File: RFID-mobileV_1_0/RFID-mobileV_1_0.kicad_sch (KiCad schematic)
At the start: 24 parts

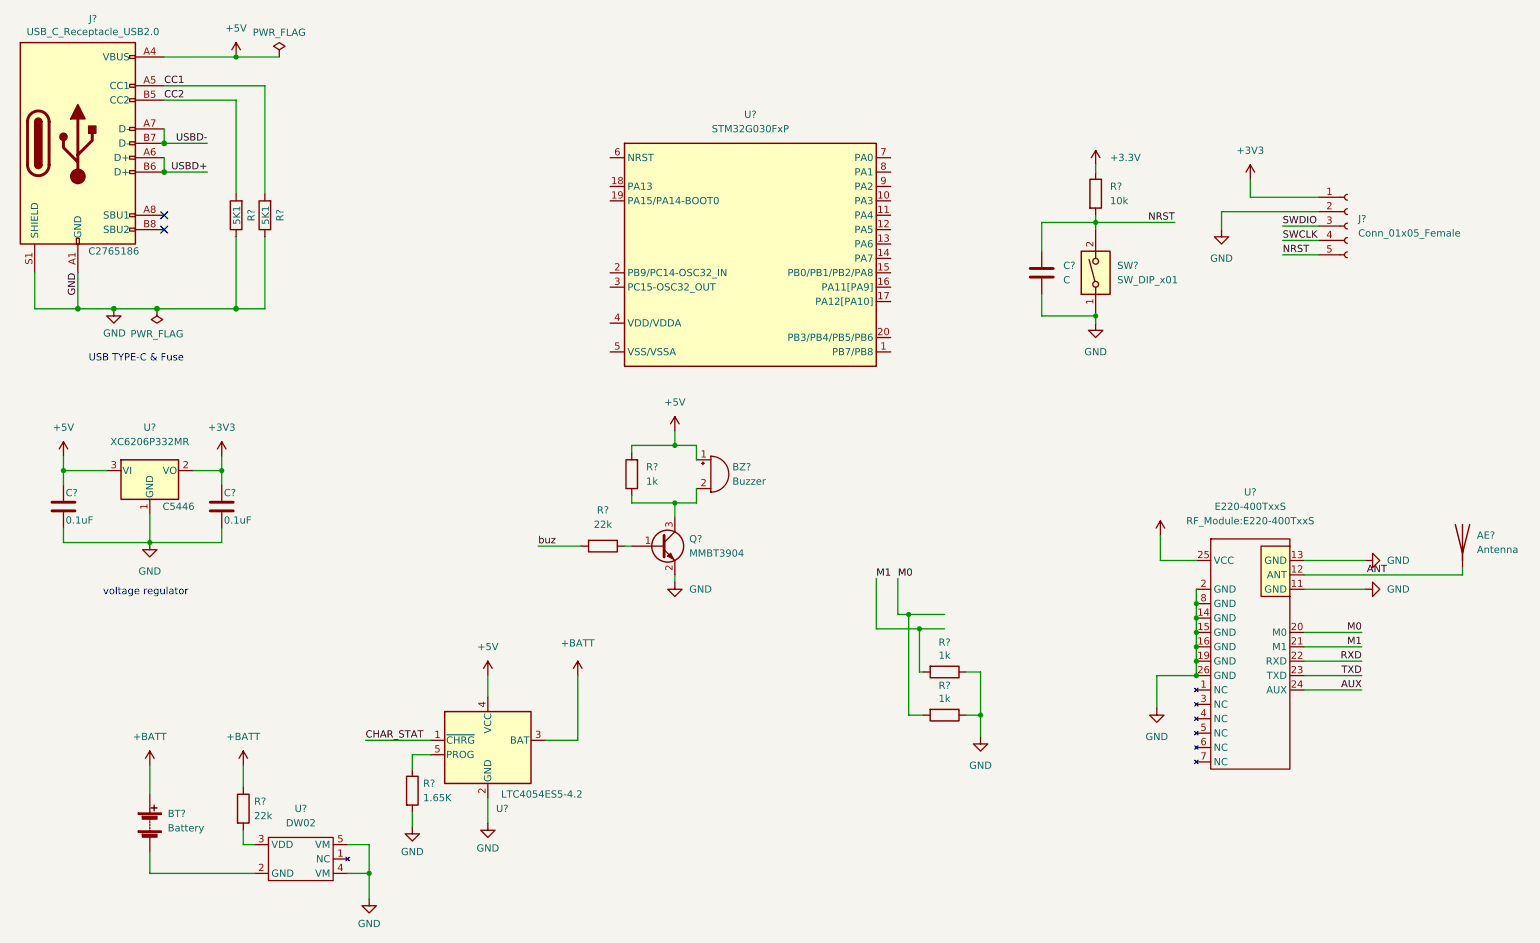
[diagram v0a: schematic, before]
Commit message: Update RFID-mobileV_1_0.kicad_sch
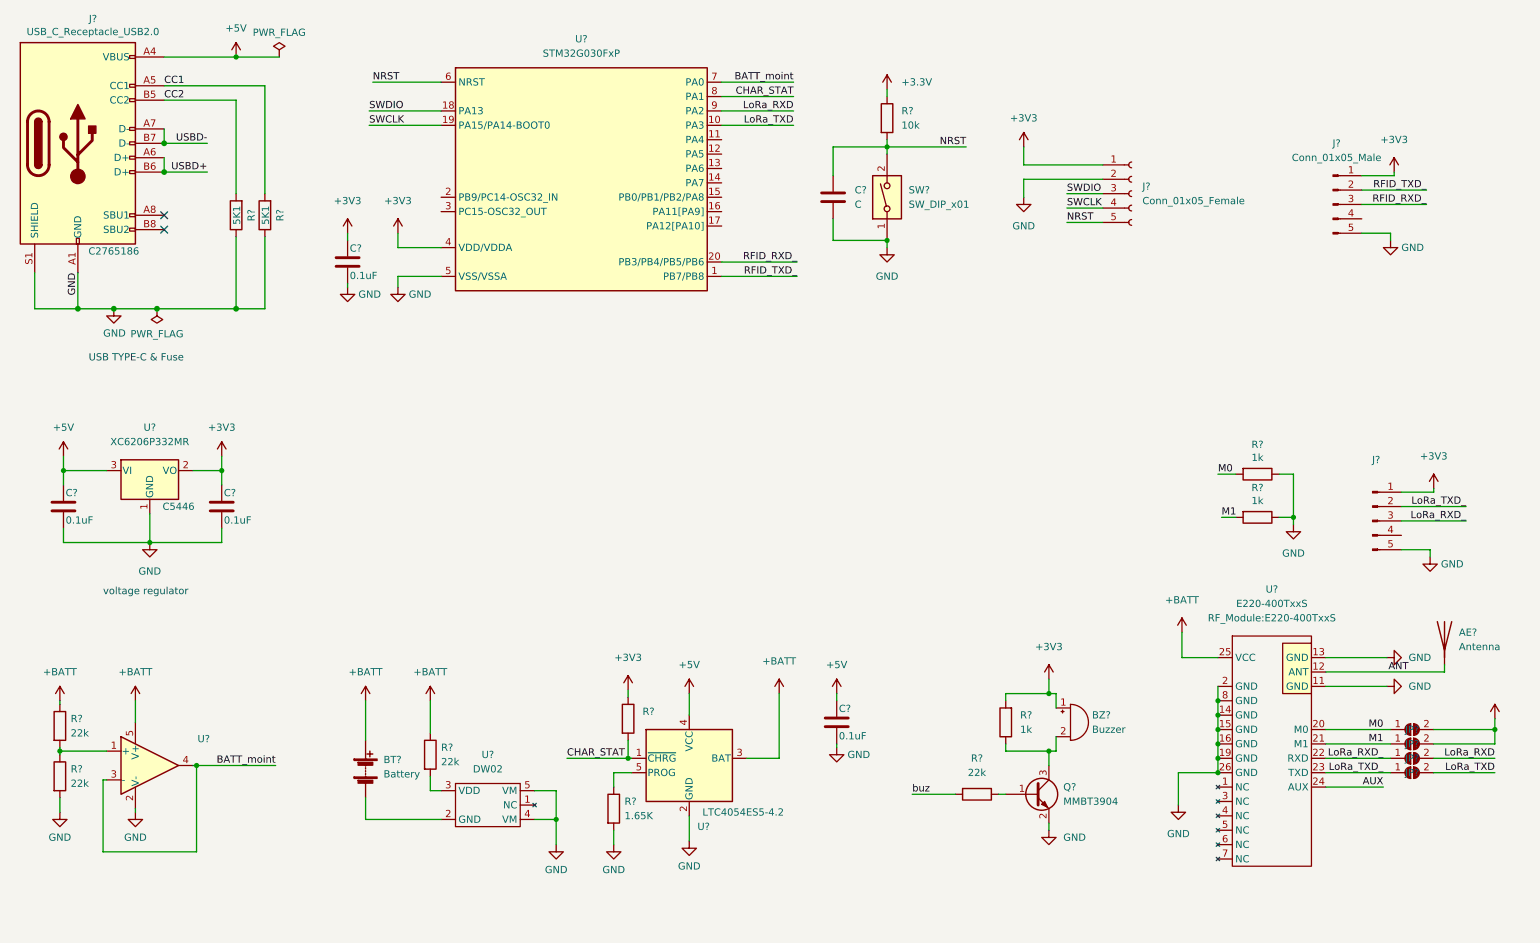
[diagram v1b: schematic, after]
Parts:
- added C? (x2): 0.1uF, Capacitor_SMD:C_0805_2012Metric, symbol Device:C
- added J?: (no value), symbol Connector:Conn_01x05_Male
- added J?: Conn_01x05_Male, Connector_PinHeader_2.54mm:PinHeader_1x05_P2.54mm_Vertical, symbol Connector:Conn_01x05_Male
- added JP? (x2): (no value), symbol Jumper:SolderJumper_2_Open
- added JP? (x2): SolderJumper_2_Open, symbol Jumper:SolderJumper_2_Open
- added R? (x2): 22k, Resistor_SMD:R_0805_2012Metric, symbol Device:R
- added R?: (no value), symbol Device:R
- added U?: (no value), symbol Amplifier_Operational:LM321
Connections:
- net +3V3: now also BZ?.1 (-), R?.2, U?.4 (VDD/VDDA), C?.1, J?.1 (Pin_1), J?.1 (Pin_1), JP?.2 (B), JP?.2 (B), R?.1
- net +5V: now also C?.1; no longer BZ?.1 (-), R?.2
- net +BATT: now also R?.1, U?.5 (V+)
- net CHAR_STAT: now also U?.8 (PA1), R?.2
- net GND: now also U?.5 (VSS/VSSA), C?.2, C?.2, J?.5 (Pin_5), J?.5 (Pin_5), R?.2, U?.2 (V-)
- net M0: now also R?.2, JP?.1 (A); no longer R?.2
- net M1: now also R?.2, JP?.1 (A); no longer R?.2
- net NRST: now also U?.6 (NRST)
- net SWCLK: now also U?.19 (PA15/PA14-BOOT0)
- net SWDIO: now also U?.18 (PA13)
- net RFID_TXD_: now reaches U?.1 (PB7/PB8)
- net RFID_TXD_: now also J?.2 (Pin_2)
- net LoRa_TXD: now reaches U?.10 (PA3)
- net LoRa_TXD: now also JP?.2 (B)
- net RFID_RXD_: now reaches U?.20 (PB3/PB4/PB5/PB6)
- net RFID_RXD_: now also J?.3 (Pin_3)
- net BATT_moint: now reaches U?.7 (PA0)
- net BATT_moint: now also U?.3 (-), U?.4
- net LoRa_RXD: now reaches U?.9 (PA2)
- net LoRa_RXD: now also JP?.2 (B)
- net RXD renamed LoRa_RXD_
- net LoRa_RXD_: now also J?.3 (Pin_3), JP?.1 (A)
- net TXD renamed LoRa_TXD_
- net LoRa_TXD_: now also J?.2 (Pin_2), JP?.1 (A)
- new net: R?.1, R?.2, U?.1 (+)
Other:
- moved on the sheet: AE?, BT?, BZ?, C?, J?, Q?, R?, SW?, U?

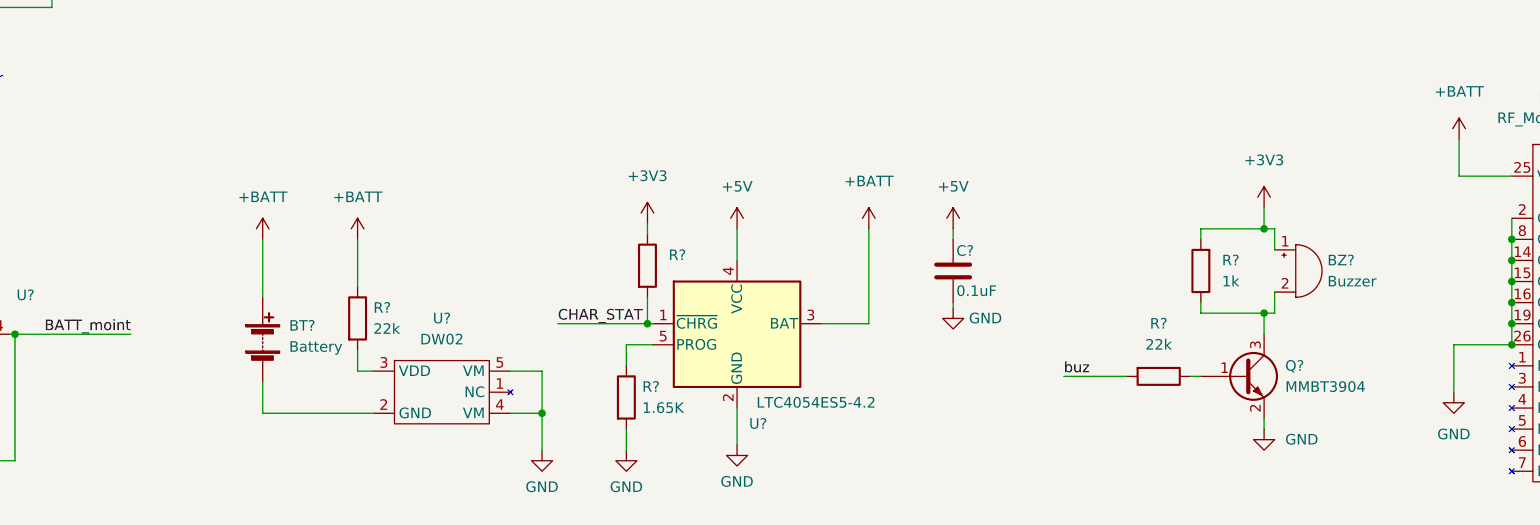
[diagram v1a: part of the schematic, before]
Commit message: Update RFID-mobileV_1_0.kicad_sch
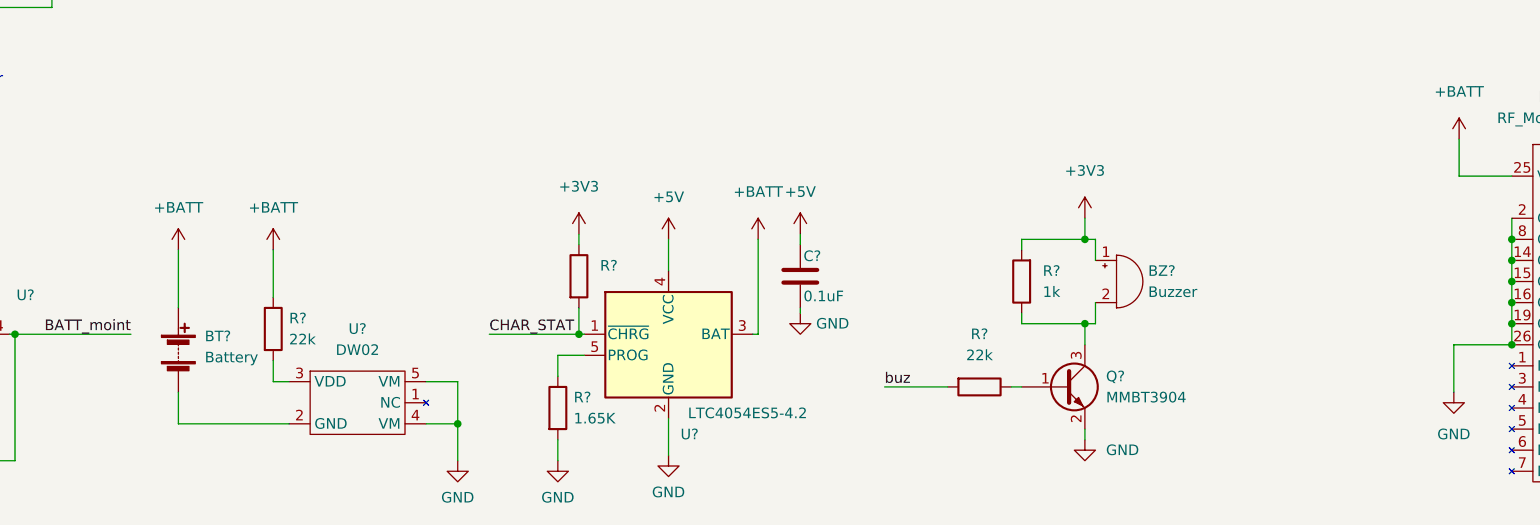
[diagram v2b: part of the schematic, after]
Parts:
- U?: LCSC (none) -> C7972
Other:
- moved on the sheet: BT?, BZ?, C?, Q?, R?, U?
